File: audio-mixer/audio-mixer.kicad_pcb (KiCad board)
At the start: 2 copper layers, 50 x 100 mm, 57 parts, among them J1 VAL**, J2 10118193-0001LF, J3 RCJ-2234, J4 SJ1-3523N, U1 PDME1-S5-D9-S, U2 MC33174, U3 MC33174, U4 MC33174

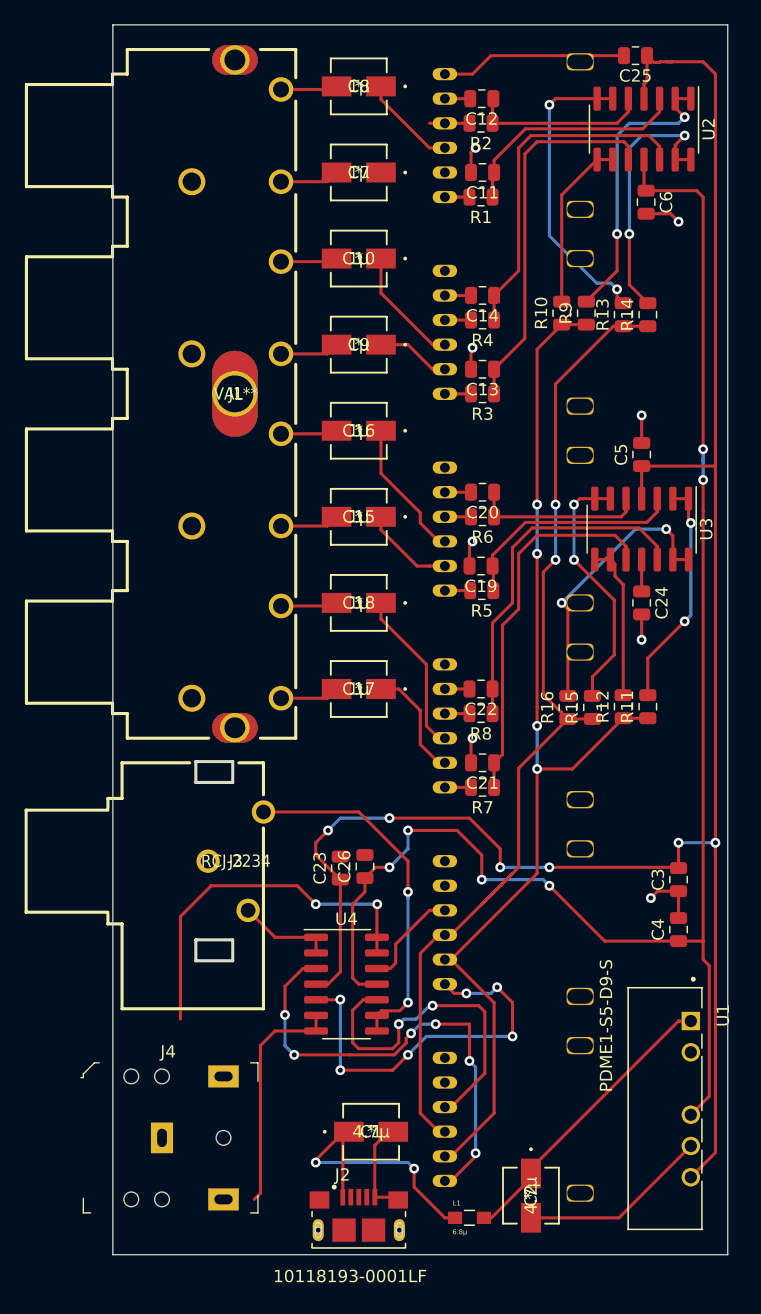
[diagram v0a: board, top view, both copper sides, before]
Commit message: updates schematic and PCB
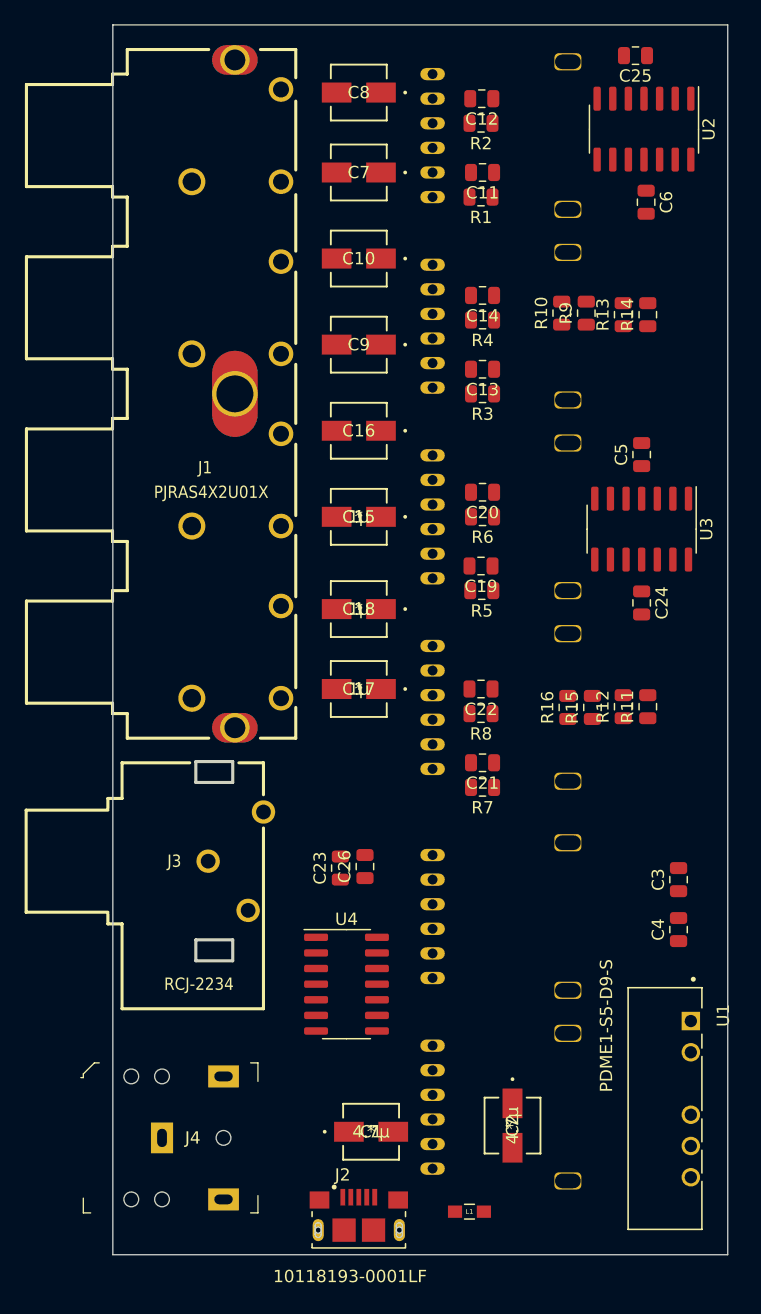
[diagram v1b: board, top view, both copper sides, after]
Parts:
- J1: value VAL** -> PJRAS4X2U01X
- moved C2 5.89 mm to (115.5, 106.5)
- moved RV4 1.80 mm to (109.0, 72.5)
- moved RV3 1.41 mm to (109.0, 57.0)
- moved RV5 1.41 mm to (109.0, 105.0)
- moved RV2 1.12 mm to (109.0, 41.5)
- moved RV6 1.12 mm to (109.0, 89.5)
- moved RV1 1.00 mm to (109.0, 26.0)
- moved C18 0.50 mm to (103.0, 64.5)
- moved C8 0.50 mm to (103.0, 22.5)
- moved L1 0.50 mm to (112.0, 113.5)
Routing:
- net +12V: track 162.3 -> 0.00 mm, vias 6 -> 0
- net -12V: track 131.4 -> 0.00 mm, vias 6 -> 0
- net MIXEDL: track 88.0 -> 0.00 mm, vias 4 -> 0
- net MIXEDR: track 83.7 -> 0.00 mm, vias 2 -> 0
- net GND: track 67.1 -> 0.00 mm, vias 8 -> 0
- net Net-(RV5-Pad2): track 38.8 -> 0.00 mm, vias 6 -> 0
- net Net-(RV6-Pad2): track 32.2 -> 0.00 mm, vias 6 -> 0
- net Net-(C21-Pad1): track 30.6 -> 0.00 mm
- net Net-(C13-Pad1): track 30.6 -> 0.00 mm
- net OUTPUT2R: track 30.0 -> 0.00 mm, vias 2 -> 0
- net OUTPUT1R: track 29.1 -> 0.00 mm, vias 2 -> 0
- net Net-(C22-Pad1): track 28.3 -> 0.00 mm
- net Net-(C14-Pad1): track 28.1 -> 0.00 mm
- net Net-(RV5-Pad5): track 27.8 -> 0.00 mm, vias 2 -> 0
- net PROC1R: track 24.6 -> 0.00 mm, vias 2 -> 0
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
